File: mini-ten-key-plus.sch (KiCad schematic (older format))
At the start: 45 parts, among them SW0 SW_Push, U0 ProMicro

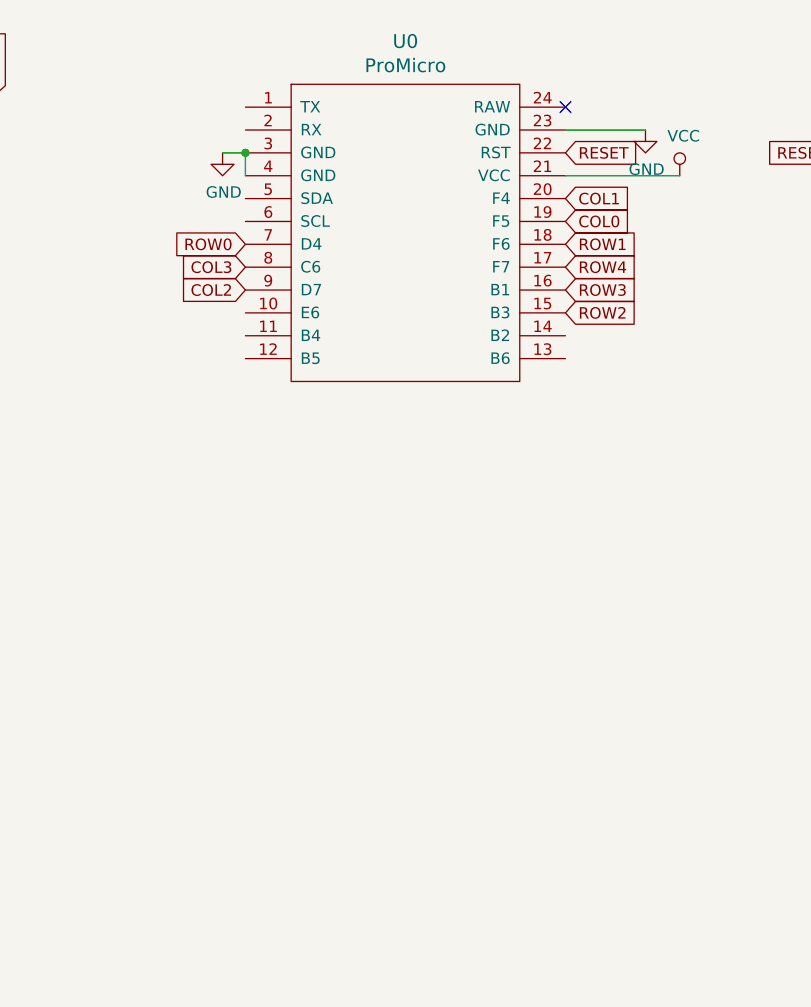
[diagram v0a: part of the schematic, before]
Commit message: General routing
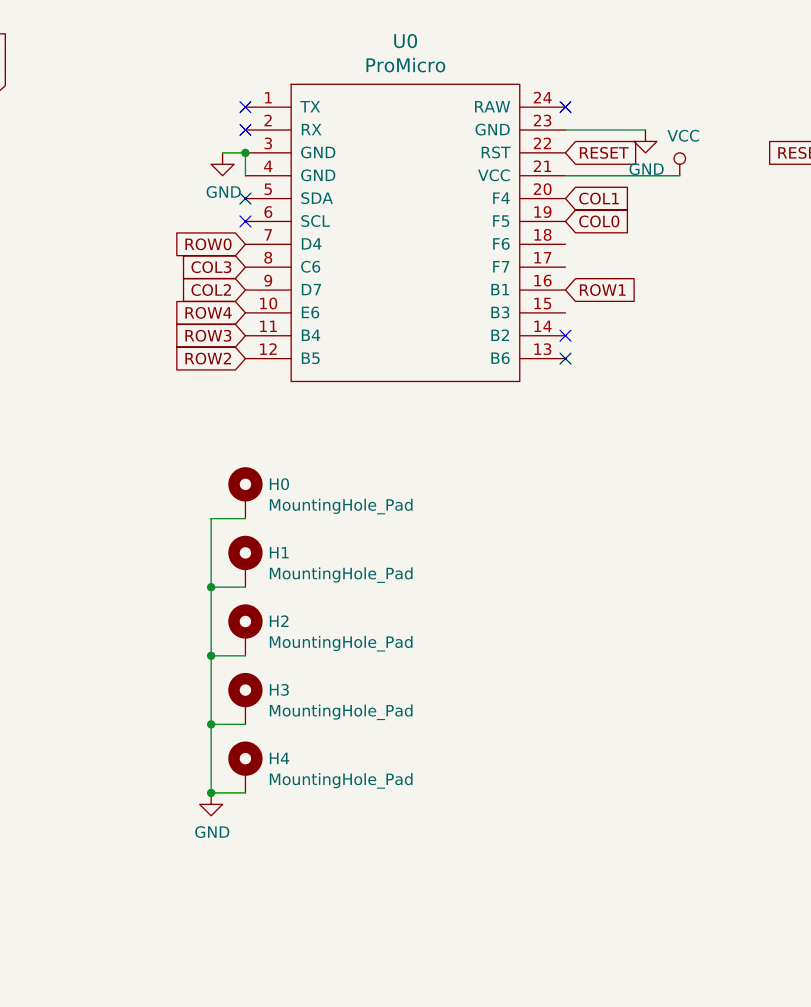
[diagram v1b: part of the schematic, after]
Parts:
- added H0, H1, H2, H3, H4: MountingHole_Pad, mini-general-tweaks:MountingHole_2.2mm_M2_Pad_tweaked, symbol Mechanical:MountingHole_Pad
- MX21: footprint mini-MX-Tweaks:MXOnly-2U-NoLED_tweak -> mini-MX-Tweaks:MXOnly-2U-NoLED_FLIPPED_tweak
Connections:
- net GND: now also H0.1, H1.1, H2.1, H3.1, H4.1
- net ROW1: now also U0.16 (B1); no longer U0.18 (F6)
- net ROW2: now also U0.12 (B5); no longer U0.15 (B3)
- net ROW3: now also U0.11 (B4); no longer U0.16 (B1)
- net ROW4: now also U0.10 (E6); no longer U0.17 (F7)
- no-connect marks 1 -> 7
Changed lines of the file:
@@
 F 0 "MX21" H 1324 3973 60  0000 C CNN
 F 1 "MX-NoLED" H 1324 3899 20  0000 C CNN
-F 2 "mini-MX-Tweaks:MXOnly-2U-NoLED_tweak" H 725 3725 60  0001 C CNN
+F 2 "mini-MX-Tweaks:MXOnly-2U-NoLED_FLIPPED_tweak" H 725 3725 60  0001 C CNN
 F 3 "" H 725 3725 60  0001 C CNN
 	1    1350 3750
@@
 Text GLabel 5050 1350 2    50   Input ~ 0
 COL0
-Text GLabel 5050 1450 2    50   Input ~ 0
+Text GLabel 5050 1650 2    50   Input ~ 0
 ROW1
 Text GLabel 3650 1450 0    50   Input ~ 0
 ROW0
-Text GLabel 5050 1750 2    50   Input ~ 0
+Text GLabel 3650 1950 0    50   Input ~ 0
 ROW2
-Text GLabel 5050 1550 2    50   Input ~ 0
+Text GLabel 3650 1750 0    50   Input ~ 0
 ROW4
-Text GLabel 5050 1650 2    50   Input ~ 0
+Text GLabel 3650 1850 0    50   Input ~ 0
 ROW3
 Text GLabel 5050 1250 2    50   Input ~ 0
@@
 Text GLabel 3650 1650 0    50   Input ~ 0
 COL2
+NoConn ~ 3650 850
+NoConn ~ 3650 950
+NoConn ~ 3650 1250
+NoConn ~ 3650 1350
+NoConn ~ 5050 1850
+NoConn ~ 5050 1950
+$Comp
+L Mechanical:MountingHole_Pad H0
+U 1 1 617941C0
+P 3650 2550
+F 0 "H0" H 3750 2599 50  0000 L CNN
+F 1 "MountingHole_Pad" H 3750 2508 50  0000 L CNN
+F 2 "mini-general-tweaks:MountingHole_2.2mm_M2_Pad_tweaked" H 3650 2550 50  0001 C CNN
+F 3 "~" H 3650 2550 50  0001 C CNN
+	1    3650 2550
+	1    0    0    -1
+$EndComp
+$Comp
+L Mechanical:MountingHole_Pad H1
+U 1 1 61795197
+P 3650 2850
+F 0 "H1" H 3750 2899 50  0000 L CNN
+F 1 "MountingHole_Pad" H 3750 2808 50  0000 L CNN
+F 2 "mini-general-tweaks:MountingHole_2.2mm_M2_Pad_tweaked" H 3650 2850 50  0001 C CNN
+F 3 "~" H 3650 2850 50  0001 C CNN
+	1    3650 2850
+	1    0    0    -1
+$EndComp
+$Comp
+L Mechanical:MountingHole_Pad H2
+U 1 1 6179748B
+P 3650 3150
+F 0 "H2" H 3750 3199 50  0000 L CNN
+F 1 "MountingHole_Pad" H 3750 3108 50  0000 L CNN
+F 2 "mini-general-tweaks:MountingHole_2.2mm_M2_Pad_tweaked" H 3650 3150 50  0001 C CNN
+F 3 "~" H 3650 3150 50  0001 C CNN
+	1    3650 3150
+	1    0    0    -1
+$EndComp
+$Comp
+L Mechanical:MountingHole_Pad H3
+U 1 1 617998EF
+P 3650 3450
+F 0 "H3" H 3750 3499 50  0000 L CNN
+F 1 "MountingHole_Pad" H 3750 3408 50  0000 L CNN
+F 2 "mini-general-tweaks:MountingHole_2.2mm_M2_Pad_tweaked" H 3650 3450 50  0001 C CNN
+F 3 "~" H 3650 3450 50  0001 C CNN
+	1    3650 3450
+	1    0    0    -1
+$EndComp
+Wire Wire Line
+	3650 2650 3500 2650
+Wire Wire Line
+	3500 2650 3500 2950
+Wire Wire Line
+	3650 3550 3500 3550
+Wire Wire Line
+	3650 3250 3500 3250
+Connection ~ 3500 3250
+Wire Wire Line
+	3500 3250 3500 3550
+Wire Wire Line
+	3650 2950 3500 2950
+Connection ~ 3500 2950
+Wire Wire Line
+	3500 2950 3500 3250
+$Comp
+L power:GND #PWR0105
+U 1 1 617A50D9
+P 3500 3850
+F 0 "#PWR0105" H 3500 3600 50  0001 C CNN
+F 1 "GND" H 3505 3677 50  0000 C CNN
+F 2 "" H 3500 3850 50  0001 C CNN
+F 3 "" H 3500 3850 50  0001 C CNN
+	1    3500 3850
+	1    0    0    -1
+$EndComp
+$Comp
+L Mechanical:MountingHole_Pad H4
+U 1 1 617BCB5D
+P 3650 3750
+F 0 "H4" H 3750 3799 50  0000 L CNN
+F 1 "MountingHole_Pad" H 3750 3708 50  0000 L CNN
+F 2 "mini-general-tweaks:MountingHole_2.2mm_M2_Pad_tweaked" H 3650 3750 50  0001 C CNN
+F 3 "~" H 3650 3750 50  0001 C CNN
+	1    3650 3750
+	1    0    0    -1
+$EndComp
+Wire Wire Line
+	3500 3550 3500 3850
+Wire Wire Line
+	3500 3850 3650 3850
+Connection ~ 3500 3550
+Connection ~ 3500 3850
 $EndSCHEMATC
